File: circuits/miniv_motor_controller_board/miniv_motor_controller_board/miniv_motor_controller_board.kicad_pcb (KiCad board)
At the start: 2 copper layers, 80 x 100 mm, 33 parts, among them J1 DC_in, J2 T200_ESC_power, J3 T200_ESC_signal, J4 Conn_EStop_Signal, SW1 SW_Push_DPDT, SW2 SW_disable_EStop, U1 Teensy4.1, U2 TLP624, U3 TLP624

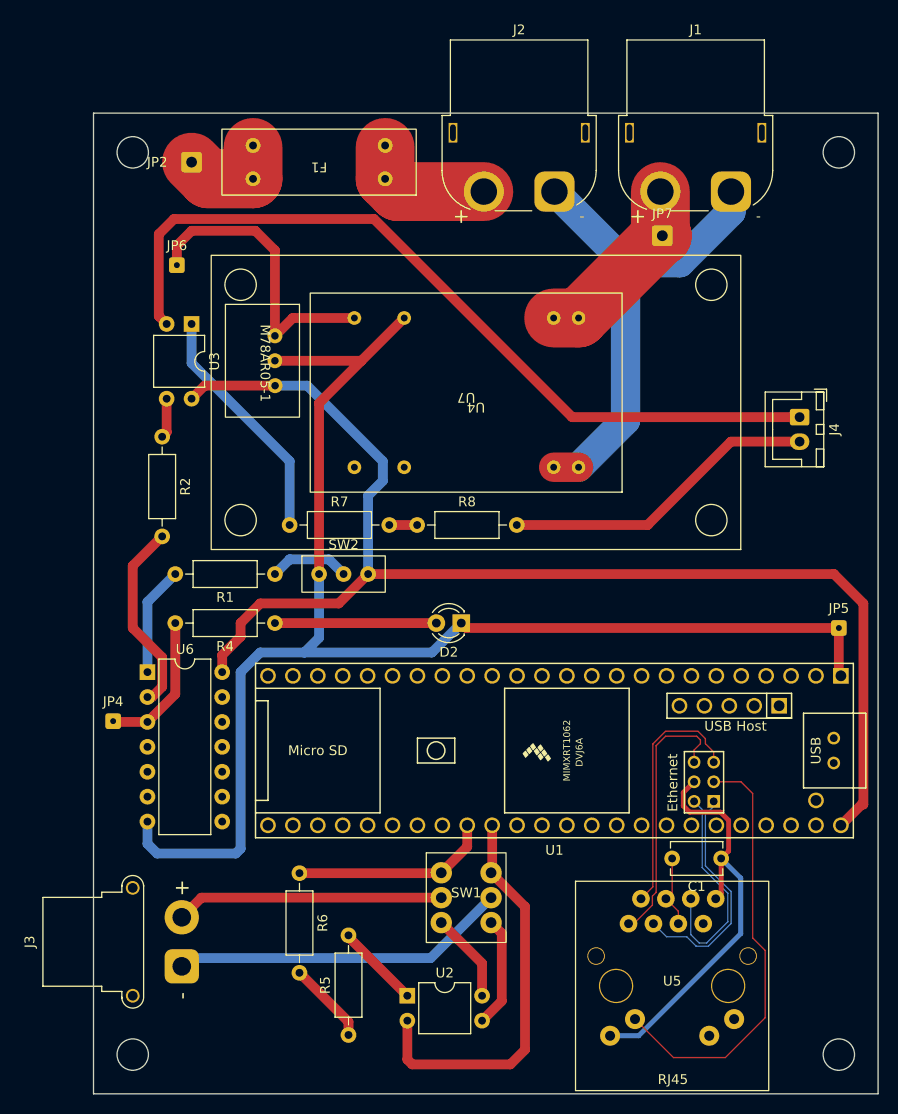
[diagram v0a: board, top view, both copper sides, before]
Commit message: add solid pattern to the board
Signed-off-by: Masaya Kataoka <ms.kataoka@gmail.com>
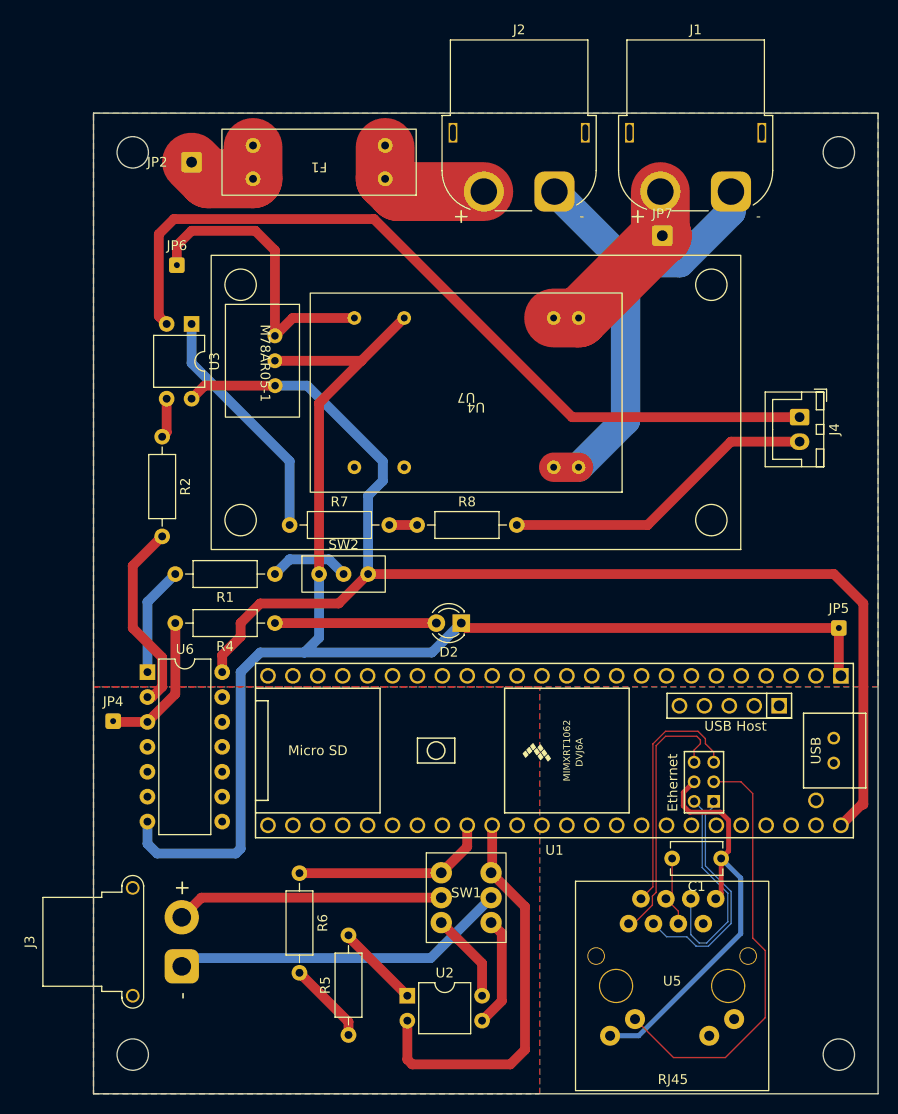
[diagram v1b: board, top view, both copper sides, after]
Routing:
- added copper zone on B.Cu, net GNDREF
- added copper zone on F.Cu, net GNDREF
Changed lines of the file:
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@@
 		(net 97)
 	)
+	(zone
+		(net 92)
+		(net_name "GNDREF")
+		(layers "F&B.Cu")
+		(hatch edge 0.5)
+		(connect_pads
+			(clearance 0.5)
+		)
+		(min_thickness 0.25)
+		(filled_areas_thickness no)
+		(fill yes
+			(thermal_gap 0.5)
+			(thermal_bridge_width 0.5)
+		)
+		(polygon
+			(pts
+				(xy 42 50) (xy 122 50) (xy 122 108.5) (xy 42 108.5)
+			)
+		)
+	)
+	(zone
+		(net 92)
+		(net_name "GNDREF")
+		(layers "F&B.Cu")
+		(hatch edge 0.5)
+		(priority 1)
+		(connect_pads
+			(clearance 0.5)
+		)
+		(min_thickness 0.25)
+		(filled_areas_thickness no)
+		(fill yes
+			(thermal_gap 0.5)
+			(thermal_bridge_width 0.5)
+		)
+		(polygon
+			(pts
+				(xy 87.5 150) (xy 87.5 108.5) (xy 42 108.5) (xy 42 150)
+			)
+		)
+	)
 )
